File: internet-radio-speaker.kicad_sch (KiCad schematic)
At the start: 32 parts, among them J1 USB-TYPE-C-018, J2 BAT_CON, Q1 DMP1045U-7, U1 USBLC6-2SC6, U101 LP4054H, U4 XC9141, U8 TPS63000

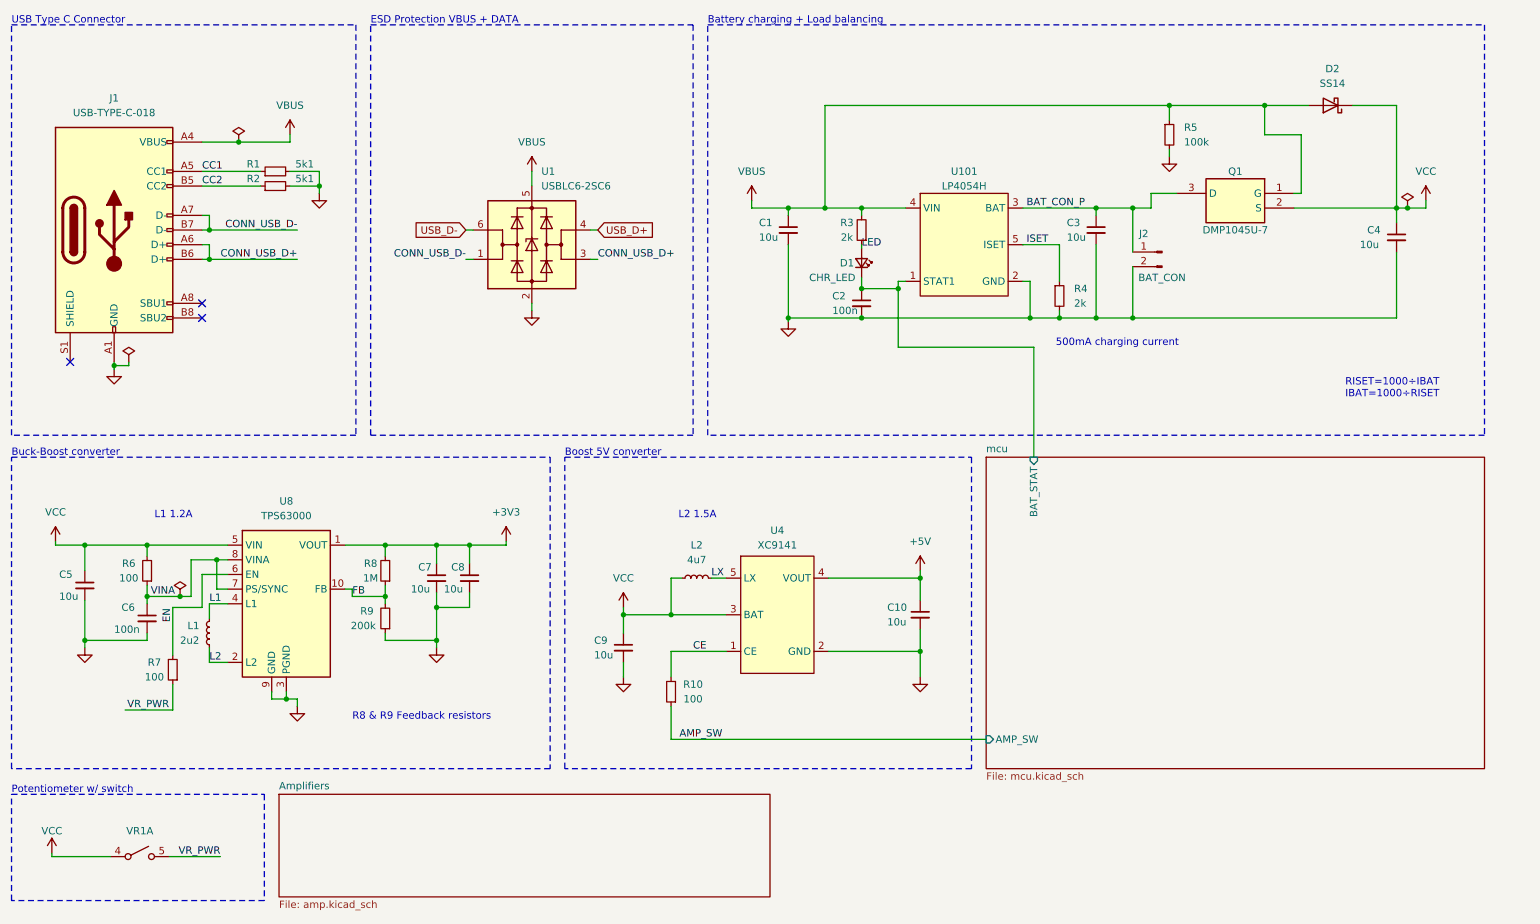
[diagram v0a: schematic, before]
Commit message: updated to rev 3
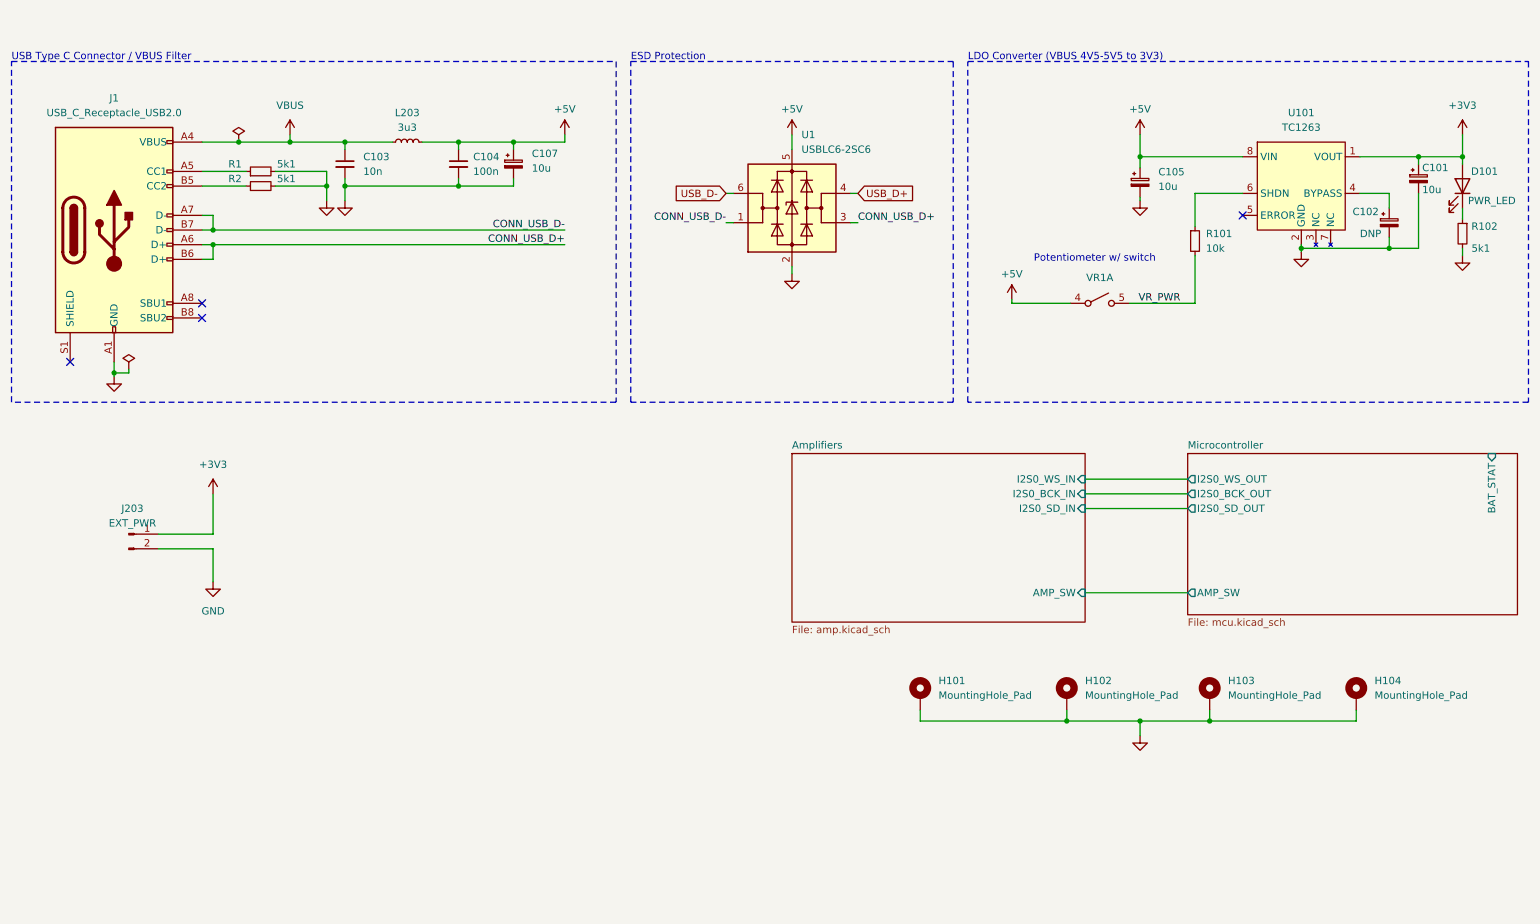
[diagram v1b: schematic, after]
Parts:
- removed C1, C10, C3, C4, C5, C7, C8, C9: 10u, Capacitor_SMD:C_0603_1608Metric, symbol Device:C_Small
- removed C2, C6: 100n, Capacitor_SMD:C_0402_1005Metric, symbol Device:C_Small
- removed D1: CHR_LED, LED_SMD:LED_0603_1608Metric, symbol Device:LED_Small
- removed D2: SS14, Diode_SMD:D_SMA, symbol Diode:B130-E3
- removed J2: BAT_CON, Connector_Wire:SolderWire-0.5sqmm_1x02_P4.6mm_D0.9mm_OD2.1mm, symbol Connector:Conn_01x02_Pin
- removed L1: 2u2, Inductor_SMD:L_0805_2012Metric, symbol Device:L_Small
- removed L2: 4u7, Inductor_SMD:L_1008_2520Metric, symbol Device:L_Small
- removed Q1: DMP1045U-7, Internet_Radio_Speaker:SOT96P240X120-3N, symbol DMP1045U-7:DMP1045U-7
- removed R10, R6, R7: 100, Resistor_SMD:R_0402_1005Metric, symbol Device:R_Small
- removed R3, R4: 2k, Resistor_SMD:R_0402_1005Metric, symbol Device:R_Small
- removed R5: 100k, Resistor_SMD:R_0402_1005Metric, symbol Device:R_Small
- removed R8: 1M, Resistor_SMD:R_0402_1005Metric, symbol Device:R_Small
- removed R9: 200k, Resistor_SMD:R_0402_1005Metric, symbol Device:R_Small
- removed U101: LP4054H, Package_TO_SOT_SMD:SOT-23-5, symbol LP4054H:LP4054H
- removed U4: XC9141, Internet_Radio_Speaker:SOT95P280X130-5N, symbol XC9141:XC9141
- removed U8: TPS63000, Package_SON:Texas_DRC0010J_ThermalVias, symbol Regulator_Switching:TPS63000
- added C101, C105, C107: 10u, Capacitor_SMD:C_0805_2012Metric, symbol Device:C_Polarized_Small
- added C102: DNP, Capacitor_SMD:C_0805_2012Metric, symbol Device:C_Polarized_Small
- added C103: 10n, Capacitor_SMD:C_0603_1608Metric, symbol Device:C_Small
- added C104: 100n, Capacitor_SMD:C_0603_1608Metric, symbol Device:C_Small
- added D101: PWR_LED, LED_SMD:LED_0805_2012Metric, symbol Device:LED
- added H101, H102, H103, H104: MountingHole_Pad, MountingHole:MountingHole_2.7mm_M2.5_DIN965_Pad, symbol Mechanical:MountingHole_Pad
- added J203: EXT_PWR, Connector_PinHeader_2.54mm:PinHeader_1x02_P2.54mm_Vertical, symbol Connector:Conn_01x02_Pin
- added L203: 3u3, Inductor_SMD:L_0805_2012Metric, symbol Device:L_Small
- added R101: 10k, Resistor_SMD:R_0603_1608Metric, symbol Device:R_Small
- added R102: 5k1, Resistor_SMD:R_0603_1608Metric, symbol Device:R_Small
- added U101: TC1263, Package_SO:SOIC-8_3.9x4.9mm_P1.27mm, symbol TC1263:TC1263
- J1: value USB-TYPE-C-018 -> USB_C_Receptacle_USB2.0; LCSC C2927038 -> (none)
- R1, R2: footprint Resistor_SMD:R_0402_1005Metric -> Resistor_SMD:R_0603_1608Metric; LCSC C25905 -> (none)
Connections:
- net VCC is gone; now on net +5V: VR1.4 (A)
- net +3V3: now also C101.1, D101.2 (A), J203.1 (Pin_1), U101.1 (VOUT)
- net +5V: now also U1.5 (VBUS), C104.1, C105.1, C107.1, L203.2, U101.8 (VIN)
- net GND: now also C101.2, C102.2, C103.2, C104.2, C105.2, C107.2, H101.1, H102.1, H103.1, H104.1, J203.2 (Pin_2), R102.2, U101.2 (GND)
- net VBUS: now also C103.1, L203.1; no longer U1.5 (VBUS)
- net VR_PWR: now also R101.2
- net CC1: no longer names the net of J1.A5 (CC1), R1.1
- net CC2: no longer names the net of J1.B5 (CC2), R2.1
- new net: C102.1, U101.4 (BYPASS)
- new net: R101.1, U101.6 (SHDN)
- new net: D101.1 (K), R102.1
- no-connect marks 3 -> 4
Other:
- sheet mcu renamed Microcontroller
- sheet Amplifiers ports: added AMP_SW, I2S0_BCK_IN, I2S0_SD_IN, I2S0_WS_IN; removed none
- sheet Microcontroller ports: added I2S0_BCK_OUT, I2S0_SD_OUT, I2S0_WS_OUT; removed none
- note added: "ESD Protection"
- note added: "LDO Converter (VBUS 4V5-5V5 to 3V3)"
- note added: "USB Type C Connector / VBUS Filter"
- note removed: "500mA charging current"
- note removed: "Battery charging + Load balancing"
- note removed: "Boost 5V converter"
- note removed: "Buck-Boost converter"
- note removed: "ESD Protection VBUS + DATA"
- note removed: "L1 1.2A"
- note removed: "L2 1.5A"
- note removed: "R8 & R9 Feedback resistors"
- note removed: "RISET=1000÷IBAT IBAT=1000÷RISET"
- note removed: "USB Type C Connector"
- moved on the sheet: U1, VR1A
